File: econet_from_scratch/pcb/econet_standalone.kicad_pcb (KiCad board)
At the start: 2 copper layers, 100 x 100 mm, 24 parts, among them CON1 jtag, U1 Econet, U2 SN65C1168, U3 LM319, U4 XC9572XL, U5 MCP1700T-3302E/MB

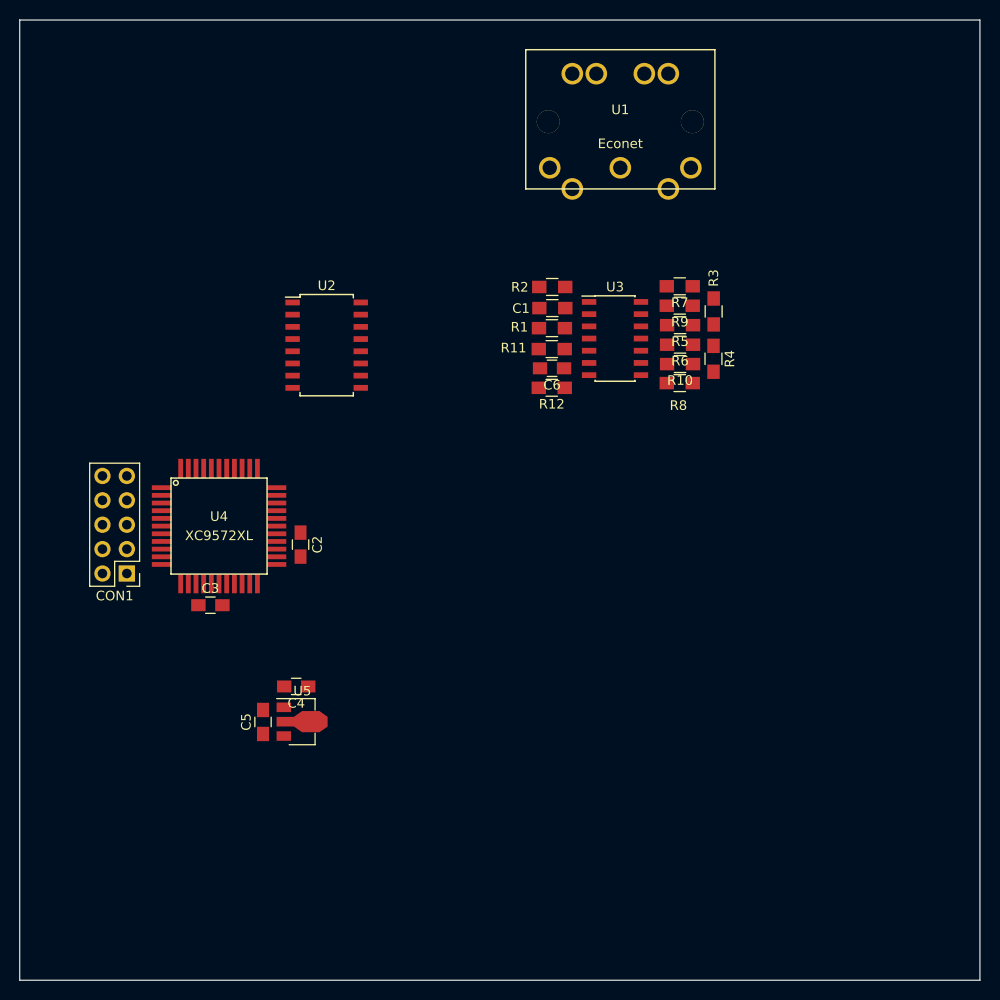
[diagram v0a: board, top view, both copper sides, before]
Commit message: More progress on econet_from_scratch
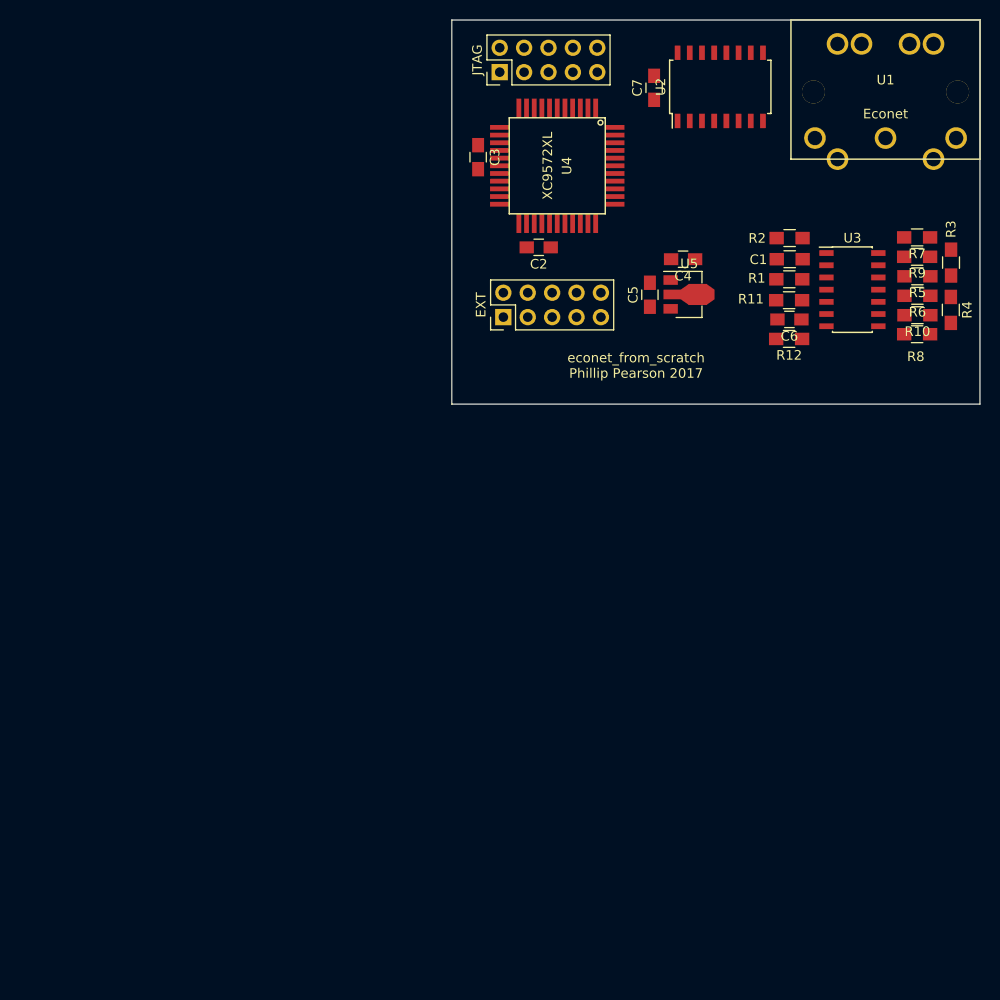
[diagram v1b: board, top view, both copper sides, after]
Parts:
- removed CON1: jtag, Pin_Headers:Pin_Header_Straight_2x05_Pitch2.54mm
- added C7: 100n, Capacitors_SMD:C_0805_HandSoldering, F.Cu at (166.1, 52.1)
- added EXT: ext, Pin_Headers:Pin_Header_Straight_2x05_Pitch2.54mm, F.Cu at (150.4, 75.9)
- added JTAG: jtag, Pin_Headers:Pin_Header_Straight_2x05_Pitch2.54mm, F.Cu at (150.0, 50.4)
- moved C4 60.0 mm to (169.1, 69.9)
- moved C5 60.0 mm to (165.6, 73.6)
- moved U5 60.0 mm to (169.3, 73.6)
- moved C3 54.4 mm to (147.7, 59.3), turned to 270 degrees
- moved U4 51.5 mm to (156.0, 60.2), turned to 270 degrees
- moved U2 49.0 mm to (173.0, 52.0), turned to 90 degrees
- moved C2 39.7 mm to (154.1, 68.7), turned to 180 degrees
- moved U1 27.8 mm to (190.2, 52.2)
- moved C1 25.2 mm to (180.2, 69.9)
- moved R1 25.2 mm to (180.2, 72.0)
- moved R10 25.2 mm to (193.5, 75.7)
- moved R12 25.2 mm to (180.1, 78.2)
- moved R2 25.2 mm to (180.2, 67.7)
- moved R4 25.2 mm to (197.0, 75.2)
- moved R5 25.2 mm to (193.5, 71.7)
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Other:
- board size 100 x 100 mm -> 55 x 40 mm
- board text added: "econet_from_scratch Phillip Pearson 2017"
